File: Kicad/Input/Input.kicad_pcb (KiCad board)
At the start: 2 copper layers, 53 x 42 mm, 37 parts, among them J1 Conn_01x02, J2 Conn_01x02, J3 Conn_01x03, U1 AD8567ARUZ, U2 MAX4016ESA+, U3 LM319

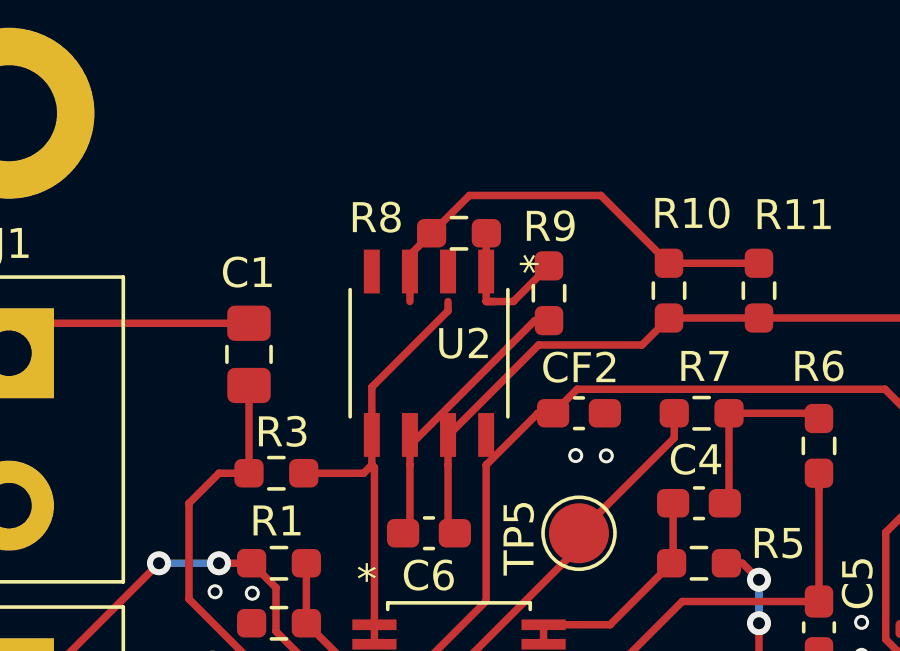
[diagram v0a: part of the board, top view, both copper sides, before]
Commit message: added gerber and drill files
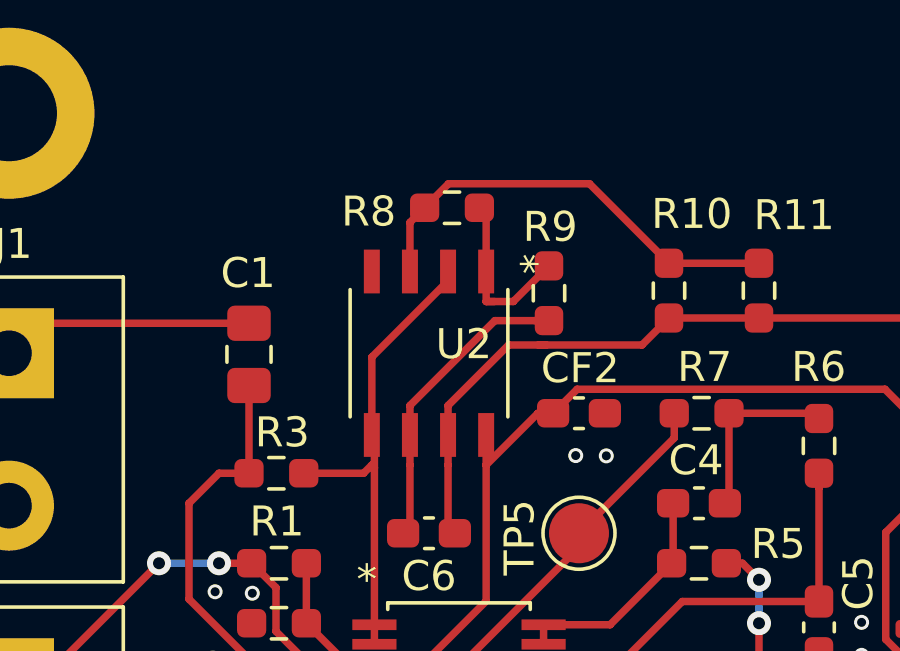
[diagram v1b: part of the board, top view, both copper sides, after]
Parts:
- moved R8 0.88 mm to (154.8, -418.9)
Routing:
- net /LPF/VREF: track 14.9 -> 16.0 mm
- net VCC: track 82.5 -> 83.5 mm
- net Net-(R8-Pad1): track 5.15 -> 6.09 mm
- net Net-(C6-Pad2): track 9.38 -> 10.3 mm
- net /Comparator/TRIANGLE_IN: track 40.7 -> 41.5 mm
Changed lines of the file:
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@@
     (thickness 1.6)
     (drawings 12)
-    (tracks 181)
+    (tracks 190)
     (zones 0)
     (modules 37)
@@
     (pcbplotparams
       (layerselection 0x010fc_ffffffff)
-      (usegerberextensions false)
-      (usegerberattributes true)
-      (usegerberadvancedattributes true)
-      (creategerberjobfile true)
+      (usegerberextensions true)
+      (usegerberattributes false)
+      (usegerberadvancedattributes false)
+      (creategerberjobfile false)
       (excludeedgelayer true)
       (linewidth 0.100000)
@@
       (psa4output false)
       (plotreference true)
-      (plotvalue true)
+      (plotvalue false)
       (plotinvisibletext false)
       (padsonsilk false)
-      (subtractmaskfromsilk false)
+      (subtractmaskfromsilk true)
       (outputformat 1)
       (mirror false)
-      (drillshape 1)
+      (drillshape 0)
       (scaleselection 1)
-      (outputdirectory ""))
+      (outputdirectory "input_gerbers"))
   )
   (net 0 "")
@@
       (effects (font (size 1 1) (thickness 0.15)))
     )
-    (fp_text user "Copyright 2021 Accelerated Designs. All rights reserved." (at 0 0 90) (layer Cmts.User)
+    (fp_text user "Copyright 2021 Accelerated Designs. All rights reserved." (at 0 0 90) (layer Cmts.User) hide
       (effects (font (size 0.127 0.127) (thickness 0.002)))
     )
@@
       (effects (font (size 1 1) (thickness 0.15)))
     )
-    (fp_text user "Copyright 2021 Accelerated Designs. All rights reserved." (at 0 0) (layer Cmts.User)
+    (fp_text user "Copyright 2021 Accelerated Designs. All rights reserved." (at 0 0) (layer Cmts.User) hide
       (effects (font (size 0.127 0.127) (thickness 0.002)))
     )
@@
   )
   (module Resistor_SMD:R_0603_1608Metric_Pad0.98x0.95mm_HandSolder (layer F.Cu)
-    (at 155 -418 180)
+    (at 154.7675 -418.85 180)
     (descr "Resistor SMD 0603 (1608 Metric), square (rectangular) end terminal, IPC_7351 nominal with elongated pad for handsoldering. (Body size source: IPC-SM-782 page 72, https://www.pcb-3d.com/wordpress/wp-content/uploads/ipc-sm-782a_amendment_1_and_2.pdf), generated with kicad-footprint-generator")
     (tags "resistor handsolder")
     (attr smd)
-    (fp_text reference R8 (at 2.76 0.5) (layer F.SilkS)
+    (fp_text reference R8 (at 2.7775 -0.13) (layer F.SilkS)
       (effects (font (size 1 1) (thickness 0.15)))
     )
@@
       (effects (font (size 0.5 0.5) (thickness 0.08)))
     )
-    (pad 2 smd roundrect (at 1.0375 0 90) (size 1.175 1.45) (layers F.Cu F.Paste F.Mask) (roundrect_rratio 0.212766)
+    (pad 2 smd roundrect (at 1.0375 0 90) (size 1.175 1.45) (layers F.Cu F.Paste F.Mask) (roundrect_rratio 0.2127659574468085)
       (net 1 /LPF/SIG_IN))
-    (pad 1 smd roundrect (at -1.0375 0 90) (size 1.175 1.45) (layers F.Cu F.Paste F.Mask) (roundrect_rratio 0.212766)
+    (pad 1 smd roundrect (at -1.0375 0 90) (size 1.175 1.45) (layers F.Cu F.Paste F.Mask) (roundrect_rratio 0.2127659574468085)
       (net 2 "Net-(C1-Pad1)"))
     (model ${KISYS3DMOD}/Capacitor_SMD.3dshapes/C_0805_2012Metric.wrl
@@
   (segment (start 153.365 -410.27585) (end 153.365 -408.2275) (width 0.25) (layer F.Cu) (net 10))
   (segment (start 153.365 -410.9275) (end 153.365 -410.27585) (width 0.25) (layer F.Cu) (net 10))
-  (segment (start 157.525 -415.0875) (end 153.365 -410.9275) (width 0.25) (layer F.Cu) (net 10))
   (segment (start 158 -415.0875) (end 157.525 -415.0875) (width 0.25) (layer F.Cu) (net 10))
+  (segment (start 156.1964 -415.0875) (end 158 -415.0875) (width 0.25) (layer F.Cu) (net 10))
+  (segment (start 153.365 -412.2561) (end 156.1964 -415.0875) (width 0.25) (layer F.Cu) (net 10))
+  (segment (start 153.365 -411.27585) (end 153.365 -412.2561) (width 0.25) (layer F.Cu) (net 10))
   (segment (start 154.635 -408.2275) (end 154.8625 -408) (width 0.25) (layer F.Cu) (net 11))
   (segment (start 154.635 -410.27585) (end 154.635 -408.2275) (width 0.25) (layer F.Cu) (net 11))
@@
   (segment (start 175.475 -402.27) (end 174.5 -402.27) (width 0.25) (layer F.Cu) (net 11))
   (segment (start 161.09999 -414.27499) (end 162 -415.175) (width 0.25) (layer F.Cu) (net 11))
-  (segment (start 157.65389 -414.27499) (end 161.09999 -414.27499) (width 0.25) (layer F.Cu) (net 11))
-  (segment (start 154.635 -411.2561) (end 157.65389 -414.27499) (width 0.25) (layer F.Cu) (net 11))
   (segment (start 154.635 -410.27585) (end 154.635 -411.2561) (width 0.25) (layer F.Cu) (net 11))
   (segment (start 170.148232 -403.54) (end 170.525 -403.54) (width 0.25) (layer F.Cu) (net 11))
@@
   (segment (start 172 -410.80449) (end 169.22499 -408.02948) (width 0.25) (layer F.Cu) (net 11))
   (segment (start 172 -414) (end 172 -410.80449) (width 0.25) (layer F.Cu) (net 11))
+  (segment (start 156.65389 -414.27499) (end 157.90499 -414.27499) (width 0.25) (layer F.Cu) (net 11))
+  (segment (start 154.635 -412.2561) (end 156.65389 -414.27499) (width 0.25) (layer F.Cu) (net 11))
+  (segment (start 154.635 -411.27585) (end 154.635 -412.2561) (width 0.25) (layer F.Cu) (net 11))
+  (segment (start 157.90499 -414.27499) (end 161.09999 -414.27499) (width 0.25) (layer F.Cu) (net 11))
+  (segment (start 157.65389 -414.27499) (end 157.90499 -414.27499) (width 0.25) (layer F.Cu) (net 11))
   (segment (start 157.62915 -412) (end 155.905 -410.27585) (width 0.25) (layer F.Cu) (net 12))
   (segment (start 158.1375 -412) (end 157.62915 -412) (width 0.25) (layer F.Cu) (net 12))
@@
   (segment (start 167.34499 -398.56249) (end 167.34499 -396.85499) (width 0.25) (layer F.Cu) (net 12))
   (segment (start 168.06 -399.2775) (end 167.34499 -398.56249) (width 0.25) (layer F.Cu) (net 12))
+  (segment (start 155.905 -410.27585) (end 155.905 -411.27585) (width 0.25) (layer F.Cu) (net 12))
   (segment (start 175.475 -406.4375) (end 174.9125 -407) (width 0.25) (layer F.Cu) (net 13))
   (segment (start 175.475 -404.81) (end 175.475 -406.4375) (width 0.25) (layer F.Cu) (net 13))
@@
   (segment (start 152.1806 -410.19025) (end 152.095 -410.27585) (width 0.25) (layer F.Cu) (net 16))
   (segment (start 152.1806 -404.950001) (end 152.1806 -410.19025) (width 0.25) (layer F.Cu) (net 16))
-  (segment (start 154.635 -415.412198) (end 154.635 -415.72415) (width 0.25) (layer F.Cu) (net 16))
-  (segment (start 152.095 -412.872198) (end 154.635 -415.412198) (width 0.25) (layer F.Cu) (net 16))
-  (segment (start 152.095 -410.27585) (end 152.095 -412.872198) (width 0.25) (layer F.Cu) (net 16))
+  (segment (start 152.1806 -411.19025) (end 152.095 -411.27585) (width 0.25) (layer F.Cu) (net 16))
+  (segment (start 152.1806 -410.19025) (end 152.1806 -411.19025) (width 0.25) (layer F.Cu) (net 16))
+  (segment (start 154.635 -416.412198) (end 154.635 -416.72415) (width 0.25) (layer F.Cu) (net 16))
+  (segment (start 152.095 -413.872198) (end 154.635 -416.412198) (width 0.25) (layer F.Cu) (net 16))
+  (segment (start 152.095 -411.27585) (end 152.095 -413.872198) (width 0.25) (layer F.Cu) (net 16))
   (segment (start 152.1806 -401.7) (end 152.1806 -401.050001) (width 0.25) (layer F.Cu) (net 17))
   (segment (start 153.1672 -401.7) (end 159 -407.5328) (width 0.25) (layer F.Cu) (net 17))
@@
   (segment (start 162.175 -411.175) (end 162.175 -412) (width 0.25) (layer F.Cu) (net 17))
   (segment (start 159 -408) (end 162.175 -411.175) (width 0.25) (layer F.Cu) (net 17))
-  (segment (start 153.365 -417.2775) (end 154.0875 -418) (width 0.25) (layer F.Cu) (net 18))
-  (segment (start 153.365 -415.72415) (end 153.365 -417.2775) (width 0.25) (layer F.Cu) (net 18))
   (segment (start 162 -417) (end 165 -417) (width 0.25) (layer F.Cu) (net 18))
   (segment (start 162 -417) (end 162 -417.01) (width 0.25) (layer F.Cu) (net 18))
   (segment (start 162 -417) (end 161.99 -417) (width 0.25) (layer F.Cu) (net 18))
-  (segment (start 161.99 -417) (end 159.73 -419.26) (width 0.25) (layer F.Cu) (net 18))
-  (segment (start 155.3475 -419.26) (end 154.0875 -418) (width 0.25) (layer F.Cu) (net 18))
-  (segment (start 159.73 -419.26) (end 155.3475 -419.26) (width 0.25) (layer F.Cu) (net 18))
-  (segment (start 155.905 -417.9925) (end 155.9125 -418) (width 0.25) (layer F.Cu) (net 19))
-  (segment (start 155.905 -415.72415) (end 155.905 -417.9925) (width 0.25) (layer F.Cu) (net 19))
+  (segment (start 153.365 -418.36) (end 153.855 -418.85) (width 0.25) (layer F.Cu) (net 18))
+  (segment (start 153.365 -416.72415) (end 153.365 -418.36) (width 0.25) (layer F.Cu) (net 18))
+  (segment (start 153.855 -418.85) (end 153.855 -418.855) (width 0.25) (layer F.Cu) (net 18))
+  (segment (start 159.34999 -419.65001) (end 162 -417) (width 0.25) (layer F.Cu) (net 18))
+  (segment (start 154.65001 -419.65001) (end 159.34999 -419.65001) (width 0.25) (layer F.Cu) (net 18))
+  (segment (start 153.855 -418.855) (end 154.65001 -419.65001) (width 0.25) (layer F.Cu) (net 18))
   (segment (start 155.905 -415.72415) (end 156.18835 -415.72415) (width 0.25) (layer F.Cu) (net 19))
   (segment (start 156.81165 -415.72415) (end 158 -416.9125) (width 0.25) (layer F.Cu) (net 19))
   (segment (start 155.905 -415.72415) (end 156.81165 -415.72415) (width 0.25) (layer F.Cu) (net 19))
+  (segment (start 155.905 -418.625) (end 155.68 -418.85) (width 0.25) (layer F.Cu) (net 19))
+  (segment (start 155.905 -415.72415) (end 155.905 -418.625) (width 0.25) (layer F.Cu) (net 19))
   (zone (net 5) (net_name GND) (layer B.Cu) (hatch edge 0.508)
     (connect_pads (clearance 0.508))
